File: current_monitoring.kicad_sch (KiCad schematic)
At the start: 0 parts

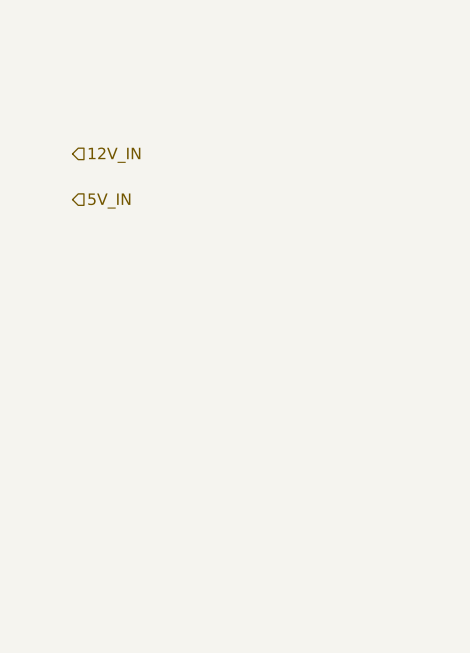
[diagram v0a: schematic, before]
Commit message: moving laptops
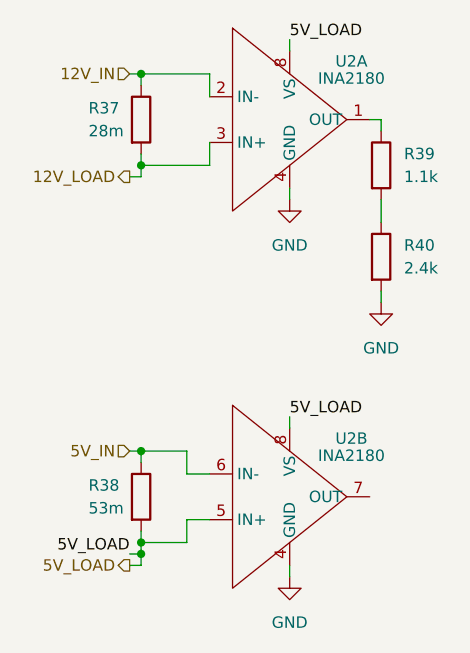
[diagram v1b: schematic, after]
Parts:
- added R37: 28m, symbol Device:R
- added R38: 53m, symbol Device:R
- added R39: 1.1k, symbol Device:R
- added R40: 2.4k, symbol Device:R
- added U2: INA2180, symbol utsvt-chips:INA2180
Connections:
- net 12V_IN: now also R37.1, U2.2 (IN-)
- net 5V_IN: now also R38.1, U2.6 (IN-)
- new net: R39.1, U2.1 (OUT)
- new net: R39.2, R40.1
- new net 12V_LOAD: R37.2, U2.3 (IN+)
- new net 5V_LOAD: R38.2, U2.5 (IN+), U2.8 (VS), U2.8 (VS)
- new net GND: R40.2, U2.4 (GND), U2.4 (GND)
